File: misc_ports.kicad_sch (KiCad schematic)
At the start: 8 parts

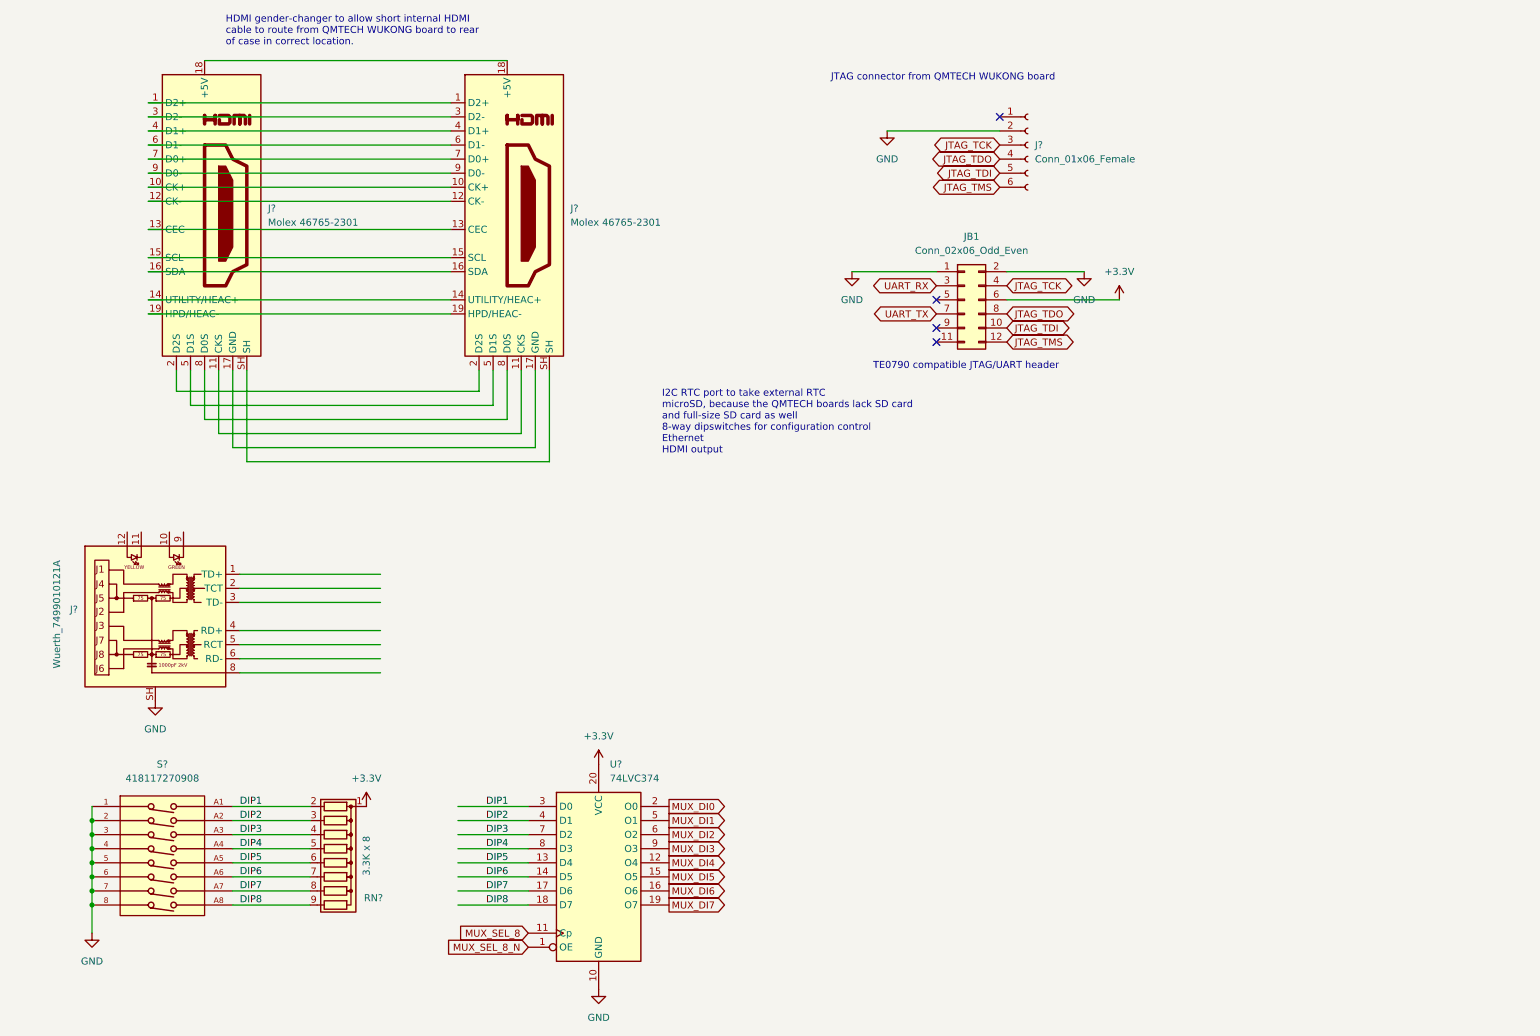
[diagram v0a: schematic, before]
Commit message: add footprint for ferrite bead, work on eth phy
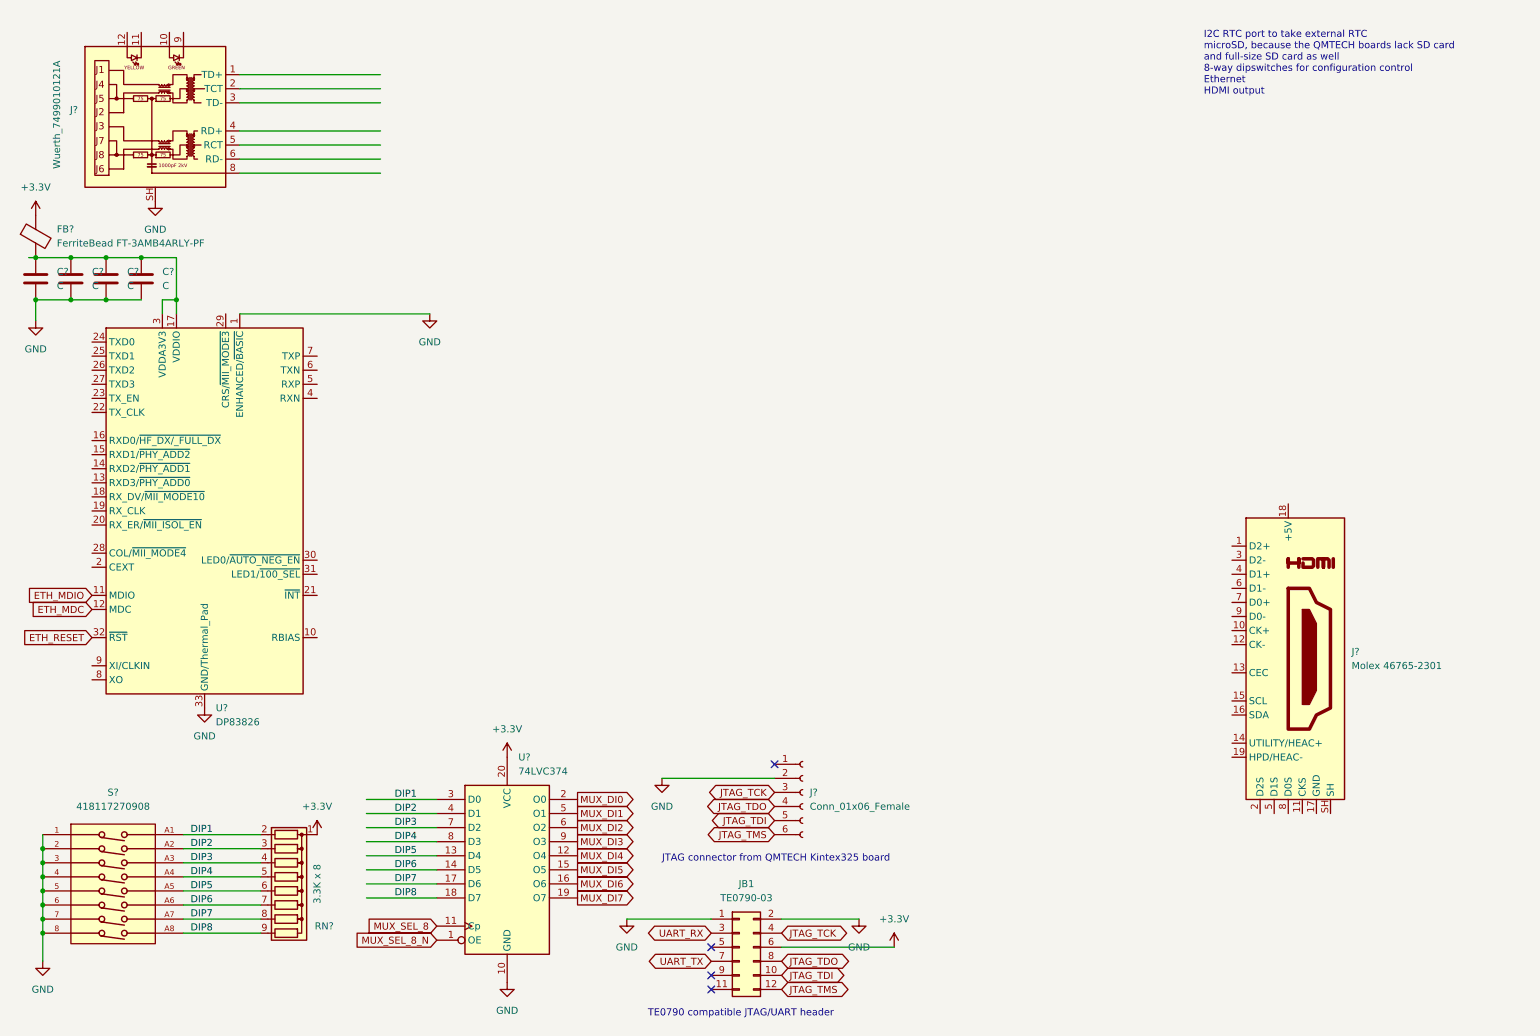
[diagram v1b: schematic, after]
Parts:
- removed J?: Molex 46765-2301, Connector_HDMI:HDMI_Micro-D_Molex_46765-2x0x, symbol Connector:HDMI_A_1.4
- added C? (x4): C, symbol Device:C
- added FB?: FerriteBead FT-3AMB4ARLY-PF, snapeda:Ferrite_Bead_Axial_L10.0mm_D4.5mm_P15.00mm_Horizontal, symbol Device:FerriteBead
- added U?: DP83826, Package_DFN_QFN:QFN-32-1EP_5x5mm_P0.5mm_EP3.3x3.3mm_ThermalVias, symbol 00Project-Eth-Phy:DP83826
- JB1: value Conn_02x06_Odd_Even -> TE0790-03
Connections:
- net +3V3: now also FB?.1
- net GND: now also C?.2, C?.2, C?.2, C?.2, U?.1 (ENHANCED/~{BASIC}), U?.33 (GND/Thermal_Pad)
- new net: C?.1, C?.1, C?.1, C?.1, FB?.2, U?.17 (VDDIO), U?.3 (VDDA3V3)
- new net ETH_MDC: U?.12 (MDC)
- new net ETH_MDIO: U?.11 (MDIO)
- new net ETH_RESET: U?.32 (~{RST})
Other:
- note added: "JTAG connector from QMTECH Kintex325 board"
- note removed: "HDMI gender-changer to allow short internal HDMI cable to route from QMTECH WUKONG board to rear of case in correct location."
- note removed: "JTAG connector from QMTECH WUKONG board"
- moved on the sheet: J?, JB1, RN?, S?, U?
